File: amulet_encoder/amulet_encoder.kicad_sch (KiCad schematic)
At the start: 46 parts, among them J7 SM07B-GHS-TB, Q7 PMV90ENER, U1 MA732GQ, U2 SN74AHC1G02DBVR

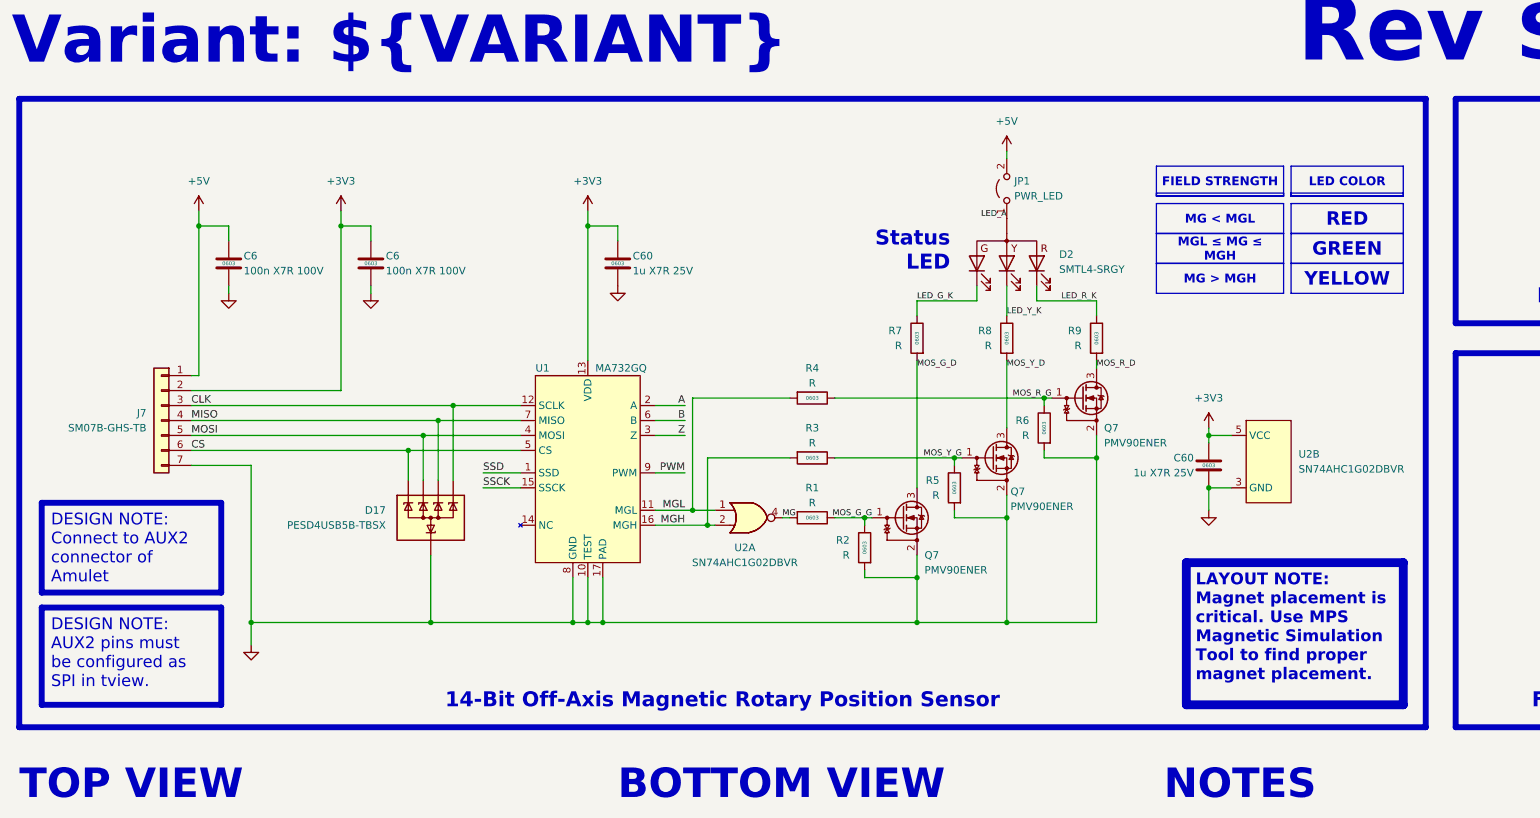
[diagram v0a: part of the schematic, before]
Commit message: rough version of encoder
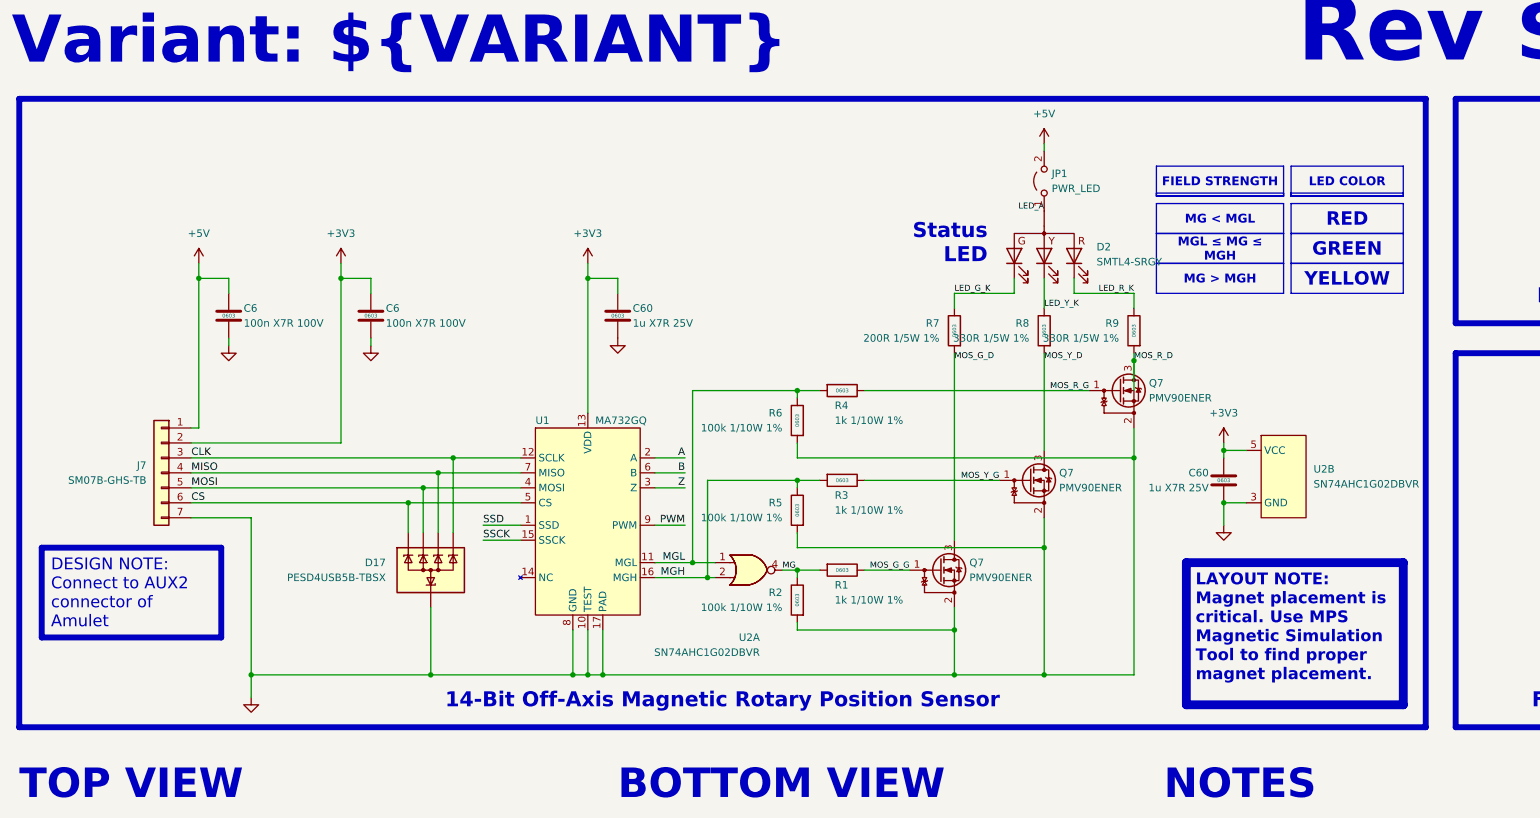
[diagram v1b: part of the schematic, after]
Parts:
- C6: Manufacturer (none) -> Taiyo Yuden; Manufacturer Part Number (none) -> HMK107B7104KAHT; Supplier 1 (none) -> Digikey; Supplier Part Number 1 (none) -> 587-6009-1-ND
- D2: Supplier 1 (none) -> Digikey; Supplier Part Number 1 (none) -> 492-2193-1-ND
- JP1: now left out of the parts list
- R1, R3, R4: value R -> 1k 1/10W 1%; Manufacturer (none) -> YAGEO; Manufacturer Part Number (none) -> RC0603FR-071KL; Supplier 1 (none) -> Digikey; Supplier Part Number 1 (none) -> 311-1.00KHRCT-ND
- R2, R5, R6: value R -> 100k 1/10W 1%; Manufacturer (none) -> YAGEO; Manufacturer Part Number (none) -> RC0603FR-07100KL; Supplier 1 (none) -> Digikey; Supplier Part Number 1 (none) -> 311-100KHRCT-ND
- R7: value R -> 200R 1/5W 1%; Manufacturer (none) -> YAGEO; Manufacturer Part Number (none) -> AC0603FR-7W200RL; Supplier 1 (none) -> Digikey; Supplier Part Number 1 (none) -> 13-AC0603FR-7W200RLCT-ND
- R8, R9: value R -> 330R 1/5W 1%; Manufacturer (none) -> TE Connectivity Passive Product; Manufacturer Part Number (none) -> CRGH0603F330R; Supplier 1 (none) -> Digikey; Supplier Part Number 1 (none) -> A129541CT-ND
- TP1: footprint 0_testpoint:TestPoint_Pad_D1mm_Front -> 0_testpoint:TestPoint_Pad_D1mm_THT
- U1: Supplier 1 (none) -> Digikey; Supplier Part Number 1 (none) -> 1589-MA732GQ-ZCT-ND
- U2: Manufacturer (none) -> Texas Instruments; Manufacturer  Texas Instruments -> (none); Supplier 1 (none) -> Digikey; Supplier Part Number 1 (none) -> 296-1088-1-ND
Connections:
- net MG: now also R2.1
- net MGH: now also R5.1
- net MGL: now also R6.1
- net MOS_G_G: no longer R2.1
- net MOS_R_G: no longer R6.1
- net MOS_Y_G: no longer R5.1
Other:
- moved on the sheet: C6, C60, D17, D2, J7, JP1, Q7, R1, R2, R3, R4, R5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
